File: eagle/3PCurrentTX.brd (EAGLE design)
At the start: 60 x 42 mm, 36 parts, among them IC1 78L05SMD, U1 SN65HVD3082ED, X1 1761543

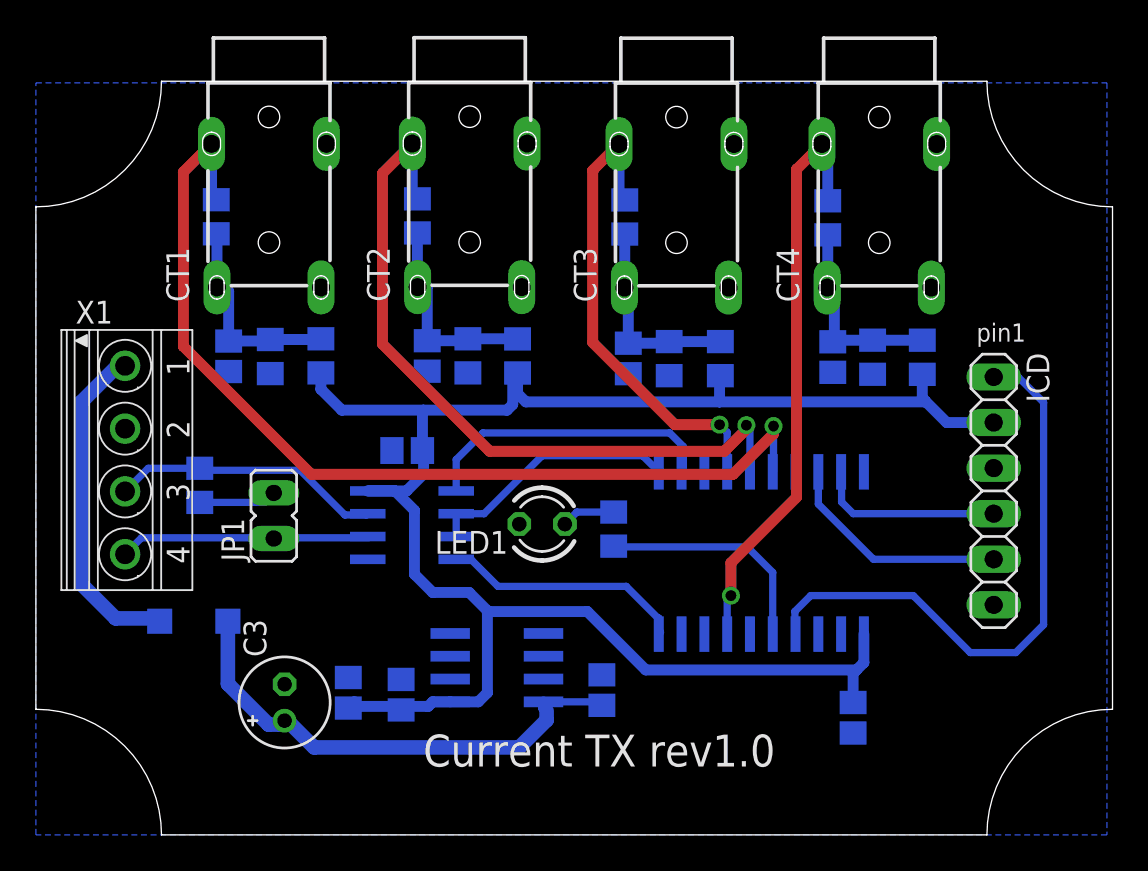
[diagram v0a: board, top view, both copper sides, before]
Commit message: Second commit of Smart EVSE
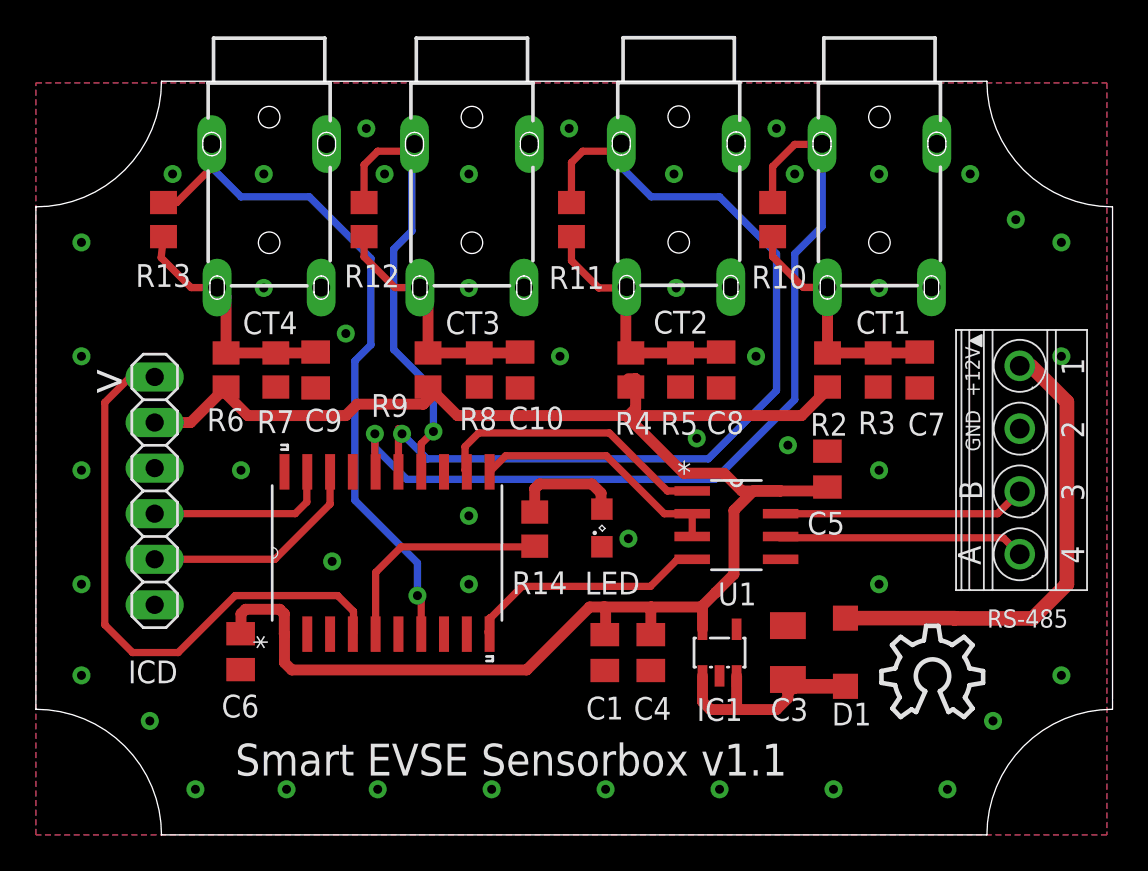
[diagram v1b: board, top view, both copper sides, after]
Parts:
- removed C2: 100n, resistor:C0805
- removed JP1: (no value), jumper:JP1
- removed LED1: 3mm, led:LED3MM
- removed R1: 120R, rcl:R0805
- removed X1: 1761543, con-phoenix-350:1751264
- added LED: (no value), led:SML0805
- added RS-485: 1761543, con-phoenix-350:1751264
- added U$2: (no value), ohw-logo:OSHW_10X200_NOTEXT
- C1, C10, C4, C5, C6, C7, C8, C9: device resistor:C0805 -> resistor:C0805K
- C3: value 47u 16v -> 10u 16v; device resistor:E2-5 -> resistor:C1206K
- D1: value 1N4148 -> LL4148
- IC1: value 78L05SMD -> LP2985IM5-5.0; device linear:SO08 -> v-reg-micrel:SOT23-5
- moved ICD 46.8 mm to (6.62, 19.2)
- moved R6 38.8 mm to (10.6, 25.9), flipped to the top
- moved C7 38.5 mm to (49.3, 25.9), flipped to the top
- moved R13 37.0 mm to (7.11, 34.3), flipped to the top
- moved D1 36.4 mm to (45.1, 10.2), flipped to the top, turned to 90 degrees
- moved C6 34.3 mm to (11.4, 10.2), flipped to the top
- moved CT1 34.0 mm to (47.0, 38.5)
- moved CT4 34.0 mm to (13.0, 38.5)
- moved R3 33.9 mm to (46.9, 25.9), flipped to the top
- moved R7 33.3 mm to (13.4, 25.9), flipped to the top
- moved R10 31.0 mm to (41.1, 34.3), flipped to the top
- moved C9 28.8 mm to (15.6, 25.9), flipped to the top
- moved R2 28.2 mm to (44.1, 25.9), flipped to the top
- moved C3 28.2 mm to (41.9, 10.2)
- moved C5 23.4 mm to (44.1, 20.4), flipped to the top, turned to 90 degrees
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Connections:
- removed net N$1: JP1.2, R1.1
- net GND: now also C3.2, LED.C, RS-485.2; no longer C2.2, C3.-, IC1.3, IC1.6, IC1.7, LED1.K, X1.2
- net N$12: now also RS-485.3; no longer R1.2, X1.3
- net N$13: now also RS-485.4; no longer JP1.1, X1.4
- net N$15: now also C3.1, IC1.1, IC1.3; no longer C2.1, C3.+, IC1.8
- net N$2: now also RS-485.1; no longer X1.1
- net N$8: now also LED.A; no longer LED1.A
- net VCC: now also IC1.5; no longer IC1.1
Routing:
- net N$15: track 28.2 -> 12.7 mm
- net N$11: track 41.2 -> 50.9 mm
- net N$2: track 18.6 -> 26.8 mm
- net N$10: track 32.8 -> 40.0 mm
- net N$7: track 54.9 -> 49.3 mm
- net N$1: track 4.61 -> 0.00 mm
- net N$8: track 3.00 -> 6.23 mm
- net N$20: track 11.3 -> 13.9 mm
- net N$18: track 11.9 -> 13.9 mm
- net N$14: track 11.9 -> 13.8 mm
- net N$21: track 12.0 -> 13.8 mm
- net N$12: track 15.4 -> 13.8 mm
- net N$4: track 16.8 -> 15.8 mm
- added copper zone on layer 1, net GND
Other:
- outline, holes or cut-outs redrawn
- board text added: "+12V"
- board text added: "100n"
- board text added: "10K"
- board text added: "10u 10v"
- board text added: "10u 16v"
- board text added: "1503_08"
- board text added: "1761543"
- board text added: "1N4148"
- board text added: "270R"
- board text added: "33R 1%"
- board text added: "3mm"
- board text added: ">"
- board text added: "A"
- board text added: "B"
- board text added: "C1"
- board text added: "C10"
- board text added: "C3"
- board text added: "C4"
- board text added: "C5"
- board text added: "C6"
- board text added: "C7"
- board text added: "C8"
- board text added: "C9"
- board text added: "CT1"
- board text added: "CT2"
- board text added: "CT3"
- board text added: "CT4"
- board text added: "D1"
- board text added: "D:/projects/stegen.com/SE_logo.bmp"
- board text added: "GND"
- board text added: "IC1"
- board text added: "ICD"
- board text added: "LED"
- board text added: "PIC18F14K22-I/SO"
- board text added: "R10"
- board text added: "R11"
- board text added: "R12"
- board text added: "R13"
- board text added: "R14"
- board text added: "R2"
- board text added: "R3"
- board text added: "R4"
- board text added: "R5"
- board text added: "R6"
- board text added: "R7"
- board text added: "R8"
- board text added: "R9"
- board text added: "RS-485"
- board text added: "SN65HVD3082ED"
- board text added: "Smart EVSE Sensorbox v1.1"
- board text added: "U1"
